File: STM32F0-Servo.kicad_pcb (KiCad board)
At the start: 2 copper layers, 99 x 69.6 mm, 106 parts, among them J1 DCC, J10 BTN_2, J11 BTN_3, J12 BTN_4, J13 LED_1, J14 LED_2, J15 LED_3, J16 LED_4, J17 SWD-DEBUG, J2 POWER, J3 BOOT, J4 TTL-SERIAL, J5 SERVO_1, J6 SERVO_2, J7 SERVO_3, J8 SERVO_4, J9 BTN_1, P1 V5-V3.3-GND, P10 PA5, P11 PA9, P12 PB4, P13 PA6, P14 PA10, P15 PB5, P16 PA7, P17 PA11, P18 PB6, P19 PA0, P2 PA3, P20 PB0, P21 PA12, P22 PB7, P23 PA1, P24 PB1, P25 PA13, P26 PA2, P27 PA14, P3 PA15, P4 PF0, P5 PA4, P6 SWO, P7 PA8, P8 PB3, P9 PF1, SW1 BUTTON PLUS, SW2 BUTTON MINUS, U1 PAM2305DABADJ, U2 6N137, U3 stm32f030-lqfp32, Y1 8MHz

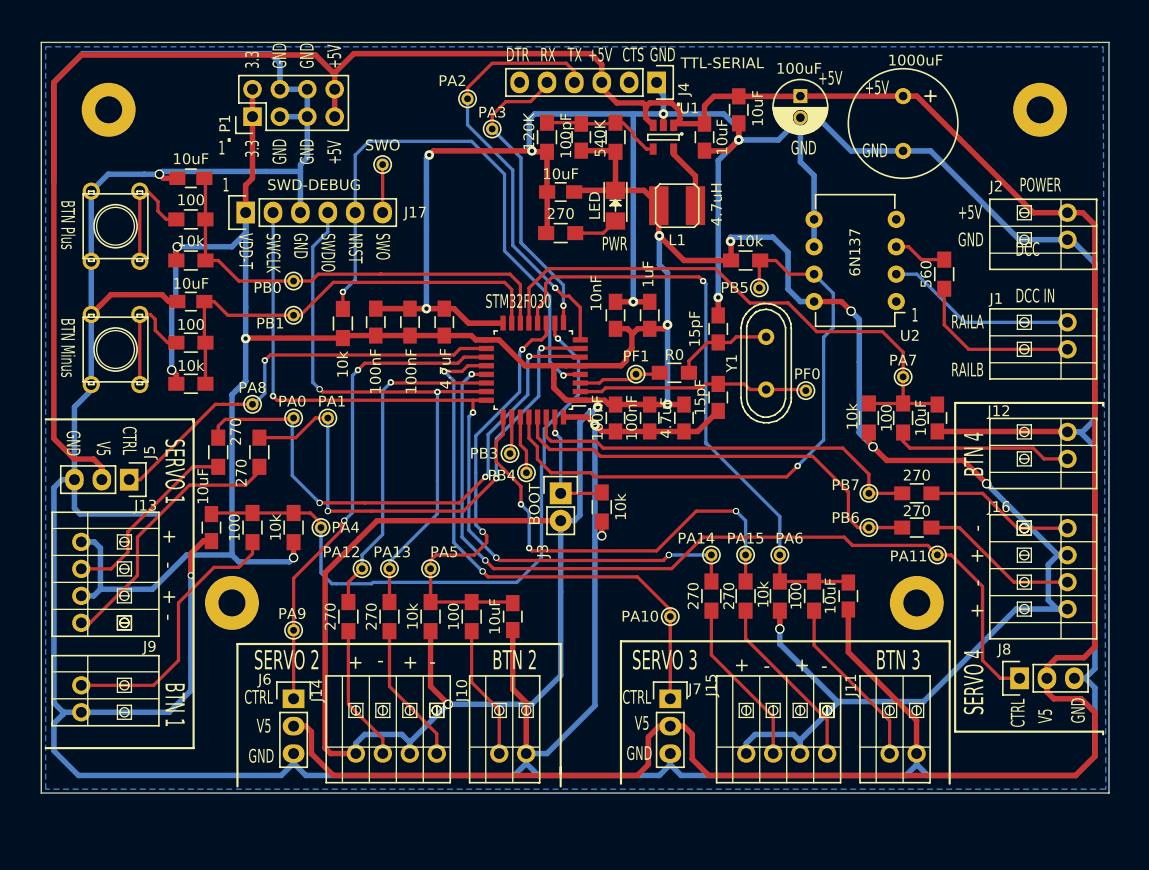
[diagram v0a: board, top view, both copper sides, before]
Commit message: Final edits for Ver 2.1, PCBs ordered from this version
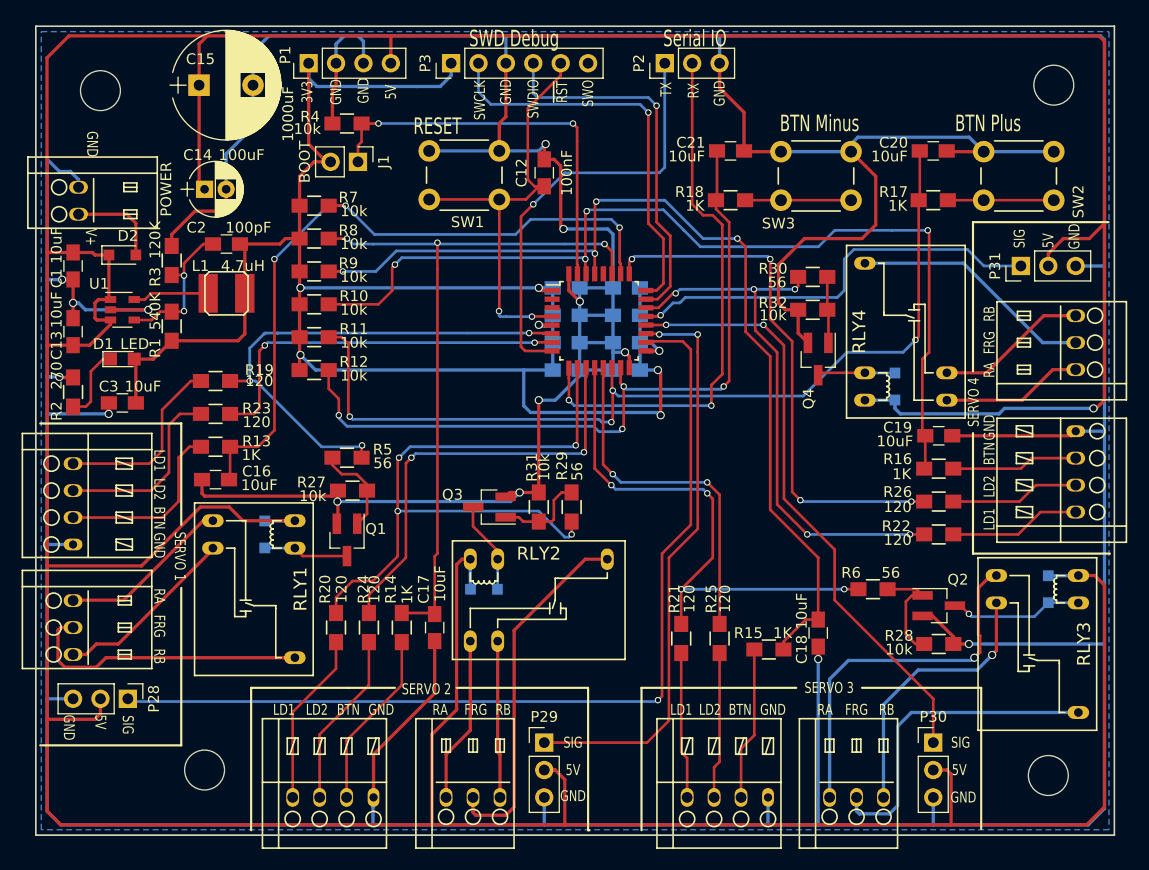
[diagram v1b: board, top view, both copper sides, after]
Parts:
- removed C22: 10uF, Capacitors_SMD:C_0805_HandSoldering
- removed J10: BTN_2, rls_misc:term_blk-phoenix-2.5mm-2
- removed J11: BTN_3, rls_misc:term_blk-phoenix-2.5mm-2
- removed J12: BTN_4, rls_misc:term_blk-phoenix-2.5mm-2
- removed J13: LED_1, rls_misc:term_blk-phoenix-2.5mm-4
- removed J14: LED_2, rls_misc:term_blk-phoenix-2.5mm-4
- removed J15: LED_3, rls_misc:term_blk-phoenix-2.5mm-4
- removed J16: LED_4, rls_misc:term_blk-phoenix-2.5mm-4
- removed J17: SWD-DEBUG, Pin_Headers:Pin_Header_Straight_1x06
- removed J3: BOOT, Pin_Headers:Pin_Header_Straight_1x02
- removed J4: TTL-SERIAL, Pin_Headers:Pin_Header_Straight_1x06
- removed J9: BTN_1, rls_misc:term_blk-phoenix-2.5mm-2
- removed P10: PA5, Connect:PINTST
- removed P11: PA9, Connect:PINTST
- removed P12: PB4, Connect:PINTST
- removed P13: PA6, Connect:PINTST
- removed P14: PA10, Connect:PINTST
- removed P15: PB5, Connect:PINTST
- removed P16: PA7, Connect:PINTST
- removed P17: PA11, Connect:PINTST
- removed P18: PB6, Connect:PINTST
- removed P19: PA0, Connect:PINTST
- removed P20: PB0, Connect:PINTST
- removed P21: PA12, Connect:PINTST
- removed P22: PB7, Connect:PINTST
- removed P23: PA1, Connect:PINTST
- removed P24: PB1, Connect:PINTST
- removed P25: PA13, Connect:PINTST
- removed P26: PA2, Connect:PINTST
- removed P27: PA14, Connect:PINTST
- removed P8: PB3, Connect:PINTST
- removed P9: PF1, Connect:PINTST
- removed the REF** at (43.2, 77.5)
- removed the REF** at (106.7, 77.5)
- removed the REF** at (118.1, 31.8)
- removed the REF** at (31.8, 31.8)
- removed U3: stm32f030-lqfp32, rls_misc:LQFP-32_7x7mm_Pitch0.8mm
- removed Y1: 8MHz, Crystals:Crystal_HC49-U_Vertical
- added D2: DIODE, Diodes_SMD:D_SOD-323_HandSoldering, F.Cu at (33.0, 45.2)
- added D3: DIODE, Diodes_SMD:D_SOD-323_HandSoldering, B.Cu at (46.2, 71.1)
- added D4: DIODE, Diodes_SMD:D_SOD-323_HandSoldering, B.Cu at (118.9, 76.2)
- added D5: DIODE, Diodes_SMD:D_SOD-323_HandSoldering, B.Cu at (66.5, 76.2)
- added D6: DIODE, Diodes_SMD:D_SOD-323_HandSoldering, B.Cu at (104.6, 57.4)
- added P28: SERVO1, Pin_Headers:Pin_Header_Straight_1x03_Pitch2.54mm, F.Cu at (33.5, 86.4)
- added P29: SERVO2, Pin_Headers:Pin_Header_Straight_1x03_Pitch2.54mm, F.Cu at (72.1, 90.4)
- added P30: SERVO3, Pin_Headers:Pin_Header_Straight_1x03_Pitch2.54mm, F.Cu at (108.2, 90.4)
- added P31: SERVO4, Pin_Headers:Pin_Header_Straight_1x03_Pitch2.54mm, F.Cu at (116.3, 46.2)
- added Q1: MMBF170, TO_SOT_Packages_SMD:SOT-23_Handsoldering, F.Cu at (53.8, 71.6)
- added Q2: MMBF170, TO_SOT_Packages_SMD:SOT-23_Handsoldering, F.Cu at (108.7, 77.7)
- added Q3: MMBF170, TO_SOT_Packages_SMD:SOT-23_Handsoldering, F.Cu at (67.1, 68.6)
- added Q4: MMBF170, TO_SOT_Packages_SMD:SOT-23_Handsoldering, F.Cu at (97.5, 54.9)
- added R29: 56, Resistors_SMD:R_0805_HandSoldering, F.Cu at (74.7, 68.6)
- added R30: 56, Resistors_SMD:R_0805_HandSoldering, F.Cu at (97.0, 47.2)
- added R31: 10k, Resistors_SMD:R_0805_HandSoldering, F.Cu at (71.6, 68.6)
- added R32: 10k, Resistors_SMD:R_0805_HandSoldering, F.Cu at (97.0, 50.3)
- added REF**: MountingHole_3.7mm, Mounting_Holes:MountingHole_3.7mm, F.Cu at (119.4, 29.5)
- added REF**: MountingHole_3.7mm, Mounting_Holes:MountingHole_3.7mm, F.Cu at (31.0, 30.0)
- added REF**: MountingHole_3.7mm, Mounting_Holes:MountingHole_3.7mm, F.Cu at (118.9, 93.5)
- added REF**: MountingHole_3.7mm, Mounting_Holes:MountingHole_3.7mm, F.Cu at (40.6, 93.0)
- added RLY1: Relay-SPDT-TE_Connectivity-Form_C, servolibrary:RELAY_SPDT, F.Cu at (45.2, 76.2)
- added RLY2: Relay-SPDT-TE_Connectivity-Form_C, servolibrary:RELAY_SPDT, F.Cu at (71.6, 77.2)
- added RLY3: Relay-SPDT-TE_Connectivity-Form_C, servolibrary:RELAY_SPDT, F.Cu at (117.9, 81.3)
- added RLY4: Relay-SPDT-TE_Connectivity-Form_C, servolibrary:RELAY_SPDT, F.Cu at (105.7, 52.3)
- added SW3: BTMINUS, Buttons_Switches_THT:SW_PUSH_6mm_h4.3mm, F.Cu at (100.6, 40.1)
- C10, C11, C4, C5, C6, C7, C8, C9: moved to B.Cu
- C12: value 10uF -> 100nF
- C13: value 100uF -> 10uF; footprint Capacitors_ThroughHole:C_Radial_D5_L11_P2 -> Capacitors_SMD:C_0805_HandSoldering
- C14: value 1000uF -> 100uF; footprint Capacitors_Elko_ThroughHole:Elko_vert_20x10mm_RM5 -> Capacitors_THT:CP_Radial_D5.0mm_P2.00mm
- C15: value 15pF -> 1000uF; footprint Capacitors_SMD:C_0805_HandSoldering -> Capacitors_THT:CP_Radial_D10.0mm_P5.00mm
- C16: value 15pF -> 10uF
- D1: footprint LEDs:LED-1206 -> LEDs:LED_0805
- J1: value DCC -> BOOT; footprint rls_misc:term_blk-phoenix-2.5mm-2 -> Pin_Headers:Pin_Header_Straight_1x02_Pitch2.54mm
- J2: footprint rls_misc:term_blk-phoenix-2.5mm-2 -> LocalLibrary:Phoenix-Combicon-2.5mm-2
- J5: value SERVO_1 -> SV1_LDBTN; footprint Pin_Headers:Pin_Header_Straight_1x03 -> LocalLibrary:Phoenix-Combicon-2.5mm-4
- J6: value SERVO_2 -> SV2_LDBTN; footprint Pin_Headers:Pin_Header_Straight_1x03 -> LocalLibrary:Phoenix-Combicon-2.5mm-4
- J7: value SERVO_3 -> SV3_LDBTN; footprint Pin_Headers:Pin_Header_Straight_1x03 -> LocalLibrary:Phoenix-Combicon-2.5mm-4
- J8: value SERVO_4 -> SV4_LDBTN; footprint Pin_Headers:Pin_Header_Straight_1x03 -> LocalLibrary:Phoenix-Combicon-2.5mm-4
- P1: value V5-V3.3-GND -> DBG POWER; footprint Pin_Headers:Pin_Header_Straight_2x04 -> Pin_Headers:Pin_Header_Straight_1x04_Pitch2.54mm
- P2: value PA3 -> SERIAL; footprint Connect:PINTST -> Pin_Headers:Pin_Header_Straight_1x03_Pitch2.54mm
- P3: value PA15 -> SWD-DEBUG; footprint Connect:PINTST -> Pin_Headers:Pin_Header_Straight_1x06_Pitch2.54mm
- P4: value PF0 -> FROG1; footprint Connect:PINTST -> LocalLibrary:Phoenix-Combicon-2.5mm-3
- P5: value PA4 -> FROG3; footprint Connect:PINTST -> LocalLibrary:Phoenix-Combicon-2.5mm-3
- P6: value SWO -> FROG4; footprint Connect:PINTST -> LocalLibrary:Phoenix-Combicon-2.5mm-3
- P7: value PA8 -> FROG2; footprint Connect:PINTST -> LocalLibrary:Phoenix-Combicon-2.5mm-3
- R1: value 10k -> 540K
- R10, R28, R9: value 100 -> 10k
- R11, R12: value 270 -> 10k
- R13, R14, R15, R16, R17, R18: value 270 -> 1K
- R19: value R0 -> 120
- R2: value 540K -> 270
- R20: value 270 -> 120
- R21, R23, R24: value 10k -> 120
- R22, R25, R26: value 100 -> 120
- R3: value 560 -> 120K
- R4: value 120K -> 10k
- R5, R6: value 10k -> 56
- SW1: value BUTTON PLUS -> Reset; footprint rls_misc:tactile-button-SPST-4.5x605mm -> Buttons_Switches_THT:SW_PUSH_6mm_h4.3mm
- SW2: value BUTTON MINUS -> BTPLUS; footprint rls_misc:tactile-button-SPST-4.5x605mm -> Buttons_Switches_THT:SW_PUSH_6mm_h4.3mm
- U1: footprint Housings_SOT-23_SOT-143_TSOT-6:SOT-23-5 -> TO_SOT_Packages_SMD:SOT-23-5
- U2: value 6N137 -> STM32F03-LQFP32; footprint Housings_DIP:DIP-8_W7.62mm -> rls_misc:LQFP-32_7x7mm_Pitch0.8mm
- moved J2 91.7 mm to (29.0, 40.1), turned to 270 degrees
- moved SW2 88.1 mm to (119.4, 40.1)
- moved R3 71.6 mm to (37.6, 45.7), turned to 90 degrees
- moved P4 71.4 mm to (28.4, 79.8), turned to 270 degrees
- moved C13 70.9 mm to (28.4, 52.3), turned to 90 degrees
- moved C20 70.2 mm to (108.2, 35.6), turned to 180 degrees
- moved J1 67.7 mm to (54.9, 36.6), turned to 270 degrees
- moved P6 66.3 mm to (121.4, 53.3), turned to 90 degrees
- moved C14 65.3 mm to (40.6, 39.1), turned to 0 degrees
- moved C1 59.8 mm to (28.4, 46.2)
- moved C18 57.1 mm to (97.5, 80.3)
- moved R25 56.2 mm to (88.4, 80.8), turned to 90 degrees
- moved C15 56.2 mm to (40.1, 29.5), turned to 0 degrees
- moved P5 55.6 mm to (101.1, 95.5)
- moved R2 55.6 mm to (28.4, 57.9), turned to 270 degrees
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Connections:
- C12 pad 1: +5V -> /NRST
- C15 pad 1: /PF0 -> +5V
- C16 pad 1: Net-(C16-Pad1) -> GND
- C16 pad 2: GND -> /BT1
- C17 pad 2: /PB0 -> /BT2
- C18 pad 2: /PA4 -> /BT3
- C19 pad 2: /PA5 -> /BT4
- C20 pad 2: /PB1 -> /BTPLUS
- C21 pad 2: /PA6 -> /BTMINUS
- D1 pad 1: +3V3 -> Net-(D1-Pad1)
- D1 pad 2: Net-(D1-Pad2) -> +3V3
- J1 pad 1: /RAILB -> /BOOT0
- J1 pad 2: /RAILA -> +3V3
- J2 pad 2: +5V -> /VIN
- J5 pad 1: /PA8 -> Net-(J5-Pad1)
- J5 pad 2: +5V -> Net-(J5-Pad2)
- J5 pad 3: GND -> /BTN1
- J6 pad 1: /PA9 -> Net-(J6-Pad1)
- J6 pad 2: +5V -> Net-(J6-Pad2)
- J6 pad 3: GND -> /BTN2
- J7 pad 1: /PA10 -> Net-(J7-Pad1)
- J7 pad 2: +5V -> Net-(J7-Pad2)
- J7 pad 3: GND -> /BTN3
- J8 pad 1: /PA11 -> Net-(J8-Pad1)
- J8 pad 2: +5V -> Net-(J8-Pad2)
- J8 pad 3: GND -> /BTN4
- P1 pad 2: +3V3 -> GND
- P1 pad 4: GND -> +5V
- P2 pad 1: /PA3 -> /TX
- P3 pad 1: /PA15 -> +3V3
- P4 pad 1: /PF0 -> /RAIL1B
- P5 pad 1: /PA4 -> /RAIL3B
- P6 pad 1: /SWO -> /RAIL4B
- P7 pad 1: /PA8 -> /RAIL2B
- R1 pad 2: /PB5 -> Net-(C2-Pad2)
- R10 pad 1: /PA4 -> +3V3
- R10 pad 2: Net-(J9-Pad1) -> /BT4
- R11 pad 1: Net-(J13-Pad2) -> +3V3
- R11 pad 2: /PA0 -> /BTPLUS
- R12 pad 1: Net-(J14-Pad2) -> +3V3
- R12 pad 2: /PA12 -> /BTMINUS
- R13 pad 1: Net-(J15-Pad2) -> /BT1
- R13 pad 2: /PA14 -> /BTN1
- R14 pad 1: Net-(J16-Pad2) -> /BT2
- R14 pad 2: /PB6 -> /BTN2
- R15 pad 1: Net-(J13-Pad4) -> /BT3
- R15 pad 2: /PA1 -> /BTN3
- R16 pad 1: Net-(J14-Pad4) -> /BT4
- R16 pad 2: /PA13 -> /BTN4
- R17 pad 1: Net-(J15-Pad4) -> /BTPLUS
- R17 pad 2: /PA15 -> Net-(R17-Pad2)
- R18 pad 1: Net-(J16-Pad4) -> /BTMINUS
- R18 pad 2: /PB7 -> Net-(R18-Pad2)
- R19 pad 1: /PF1 -> Net-(J5-Pad1)
- R19 pad 2: Net-(C16-Pad1) -> /LD1A
- R2 pad 1: +3V3 -> GND
- R2 pad 2: Net-(C2-Pad2) -> Net-(D1-Pad1)
- R20 pad 1: GND -> Net-(J6-Pad1)
- R20 pad 2: Net-(D1-Pad2) -> /LD2A
- R21 pad 1: +3V3 -> Net-(J7-Pad1)
- R21 pad 2: /PA5 -> /LD3A
- R22 pad 1: /PA5 -> Net-(J8-Pad1)
- R22 pad 2: Net-(J10-Pad1) -> /LD4A
- R23 pad 1: +3V3 -> Net-(J5-Pad2)
- R23 pad 2: /PB1 -> /LD1B
- R24 pad 1: +3V3 -> Net-(J6-Pad2)
- R24 pad 2: /PA6 -> /LD2B
- R25 pad 1: /PB1 -> Net-(J7-Pad2)
- R25 pad 2: Net-(R25-Pad2) -> /LD3B
- R26 pad 1: /PA6 -> Net-(J8-Pad2)
- R26 pad 2: Net-(J11-Pad1) -> /LD4B
- R27 pad 1: +3V3 -> Net-(Q1-Pad1)
- R27 pad 2: /PA7 -> GND
- R28 pad 1: /PA7 -> Net-(Q2-Pad1)
- R28 pad 2: Net-(J12-Pad1) -> GND
- R3 pad 1: Net-(R3-Pad1) -> Net-(C2-Pad2)
- R3 pad 2: /RAILB -> GND
- R4 pad 1: Net-(C2-Pad2) -> /BOOT0
- R5 pad 1: /BOOT0 -> Net-(Q1-Pad1)
- R5 pad 2: GND -> /LD1A
- R6 pad 1: +3V3 -> Net-(Q2-Pad1)
- R6 pad 2: /NRST -> /LD3A
- R7 pad 2: /PB0 -> /BT1
- R8 pad 2: /PA4 -> /BT2
- R9 pad 1: /PB0 -> +3V3
- R9 pad 2: Net-(R9-Pad2) -> /BT3
- SW1 pad 2: GND -> /NRST
- SW2 pad 1: GND -> Net-(R17-Pad2)
- U2 pad 1: Net-(U2-Pad1) -> +3V3
- U2 pad 2: /RAILA -> /PF0
- U2 pad 3: Net-(R3-Pad1) -> /PF1
- U2 pad 4: Net-(U2-Pad4) -> /NRST
- U2 pad 5: GND -> +3V3
- U2 pad 6: GND -> /LD1A
- U2 pad 7: /PB5 -> /LD1B
- U2 pad 8: +3V3 -> /TX
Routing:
- net +3V3: track 412.2 -> 170.4 mm, vias 14 -> 7
- net +5V: track 299.2 -> 476.1 mm, vias 0 -> 1
- net /BT3: track 0.00 -> 90.2 mm, vias 0 -> 4
- net /BT4: track 0.00 -> 89.1 mm, vias 0 -> 4
- net /SV1: track 0.00 -> 87.6 mm, vias 0 -> 1
- net /BTPLUS: track 0.00 -> 86.6 mm, vias 0 -> 4
- net /PA11: track 80.4 -> 0.00 mm, vias 2 -> 0
- net /PA14: track 75.5 -> 0.00 mm, vias 4 -> 0
- net /BTMINUS: track 0.00 -> 69.9 mm, vias 0 -> 4
- net /BT2: track 0.00 -> 66.6 mm, vias 0 -> 3
- net GND: track 592.4 -> 658.7 mm, vias 11 -> 14
- net /BT1: track 0.00 -> 65.7 mm, vias 0 -> 3
- net /PA4: track 61.2 -> 0.00 mm, vias 1 -> 0
- net /LD2A: track 0.00 -> 60.5 mm, vias 0 -> 4
- net /PB5: track 57.4 -> 0.00 mm, vias 1 -> 0
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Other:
- board size 99 x 69.6 mm -> 100 x 75 mm
- net class Default: clearance 0.254 -> 0.2; trace_width 0.3048 -> 0.25
- net class POWER: trace_width 0.508 -> 0.3048; via_dia 0.889 -> 0.762; via_drill 0.635 -> 0.5588
- net class POWER5V removed
- rule pad_to_mask_clearance: 0 -> 0.2
- rule trace_clearance: 0.254 -> 0.2
- rule trace_min: 0.3048 -> 0.2
- board text added: "3V3"
- board text added: "5V"
- board text added: "BTN"
- board text added: "FRG"
- board text added: "LD1"
- board text added: "LD2"
- board text added: "Model Railroad Turnout Controller - Version 2.1 Original Design by Randy Stockberger - Drives up to 4 RC Servos - Frog polarity controlled via SPDT relays - Turnout positions determined via switches - Two status LED for each turnout - BTN Plus and BTN Minus feedback buttons to fine tune the servo resting positions"
- board text added: "RA"
- board text added: "RB"
- board text added: "RESET"
- board text added: "SIG"
- board text added: "SWD Debug"
- board text added: "Serial IO"
- board text added: "V+"
- board text added: "~RST"
- board text removed: "(C) 2016, Randy Stockberger Open Source Use at your own risk"
- board text removed: "+"
- board text removed: "+5V"
- board text removed: "-"
- board text removed: "."
- board text removed: "1"
- board text removed: "3.3"
- board text removed: "BTN 1"
- board text removed: "BTN 2"
- board text removed: "BTN 3"
- board text removed: "BTN 4"
- board text removed: "CTRL"
- board text removed: "CTS"
- board text removed: "DCC"
- board text removed: "DCC IN"
- board text removed: "DTR"
- board text removed: "NRST"
- board text removed: "POWER"
- board text removed: "PWR"
- board text removed: "RAILA"
- board text removed: "RAILB"
- board text removed: "STM32-Servo Ver 2.0 June, 2016"
- board text removed: "STM32F030"
- board text removed: "STM32F030 servo turnout controller for model railroads (C) 2016 Randy Stockberger This design may be used by any person for any purpose. This design has not been tested. Use at your own risk."
- board text removed: "V5"
- board text removed: "VDD-T"
